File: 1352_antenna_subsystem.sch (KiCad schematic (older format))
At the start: 24 parts

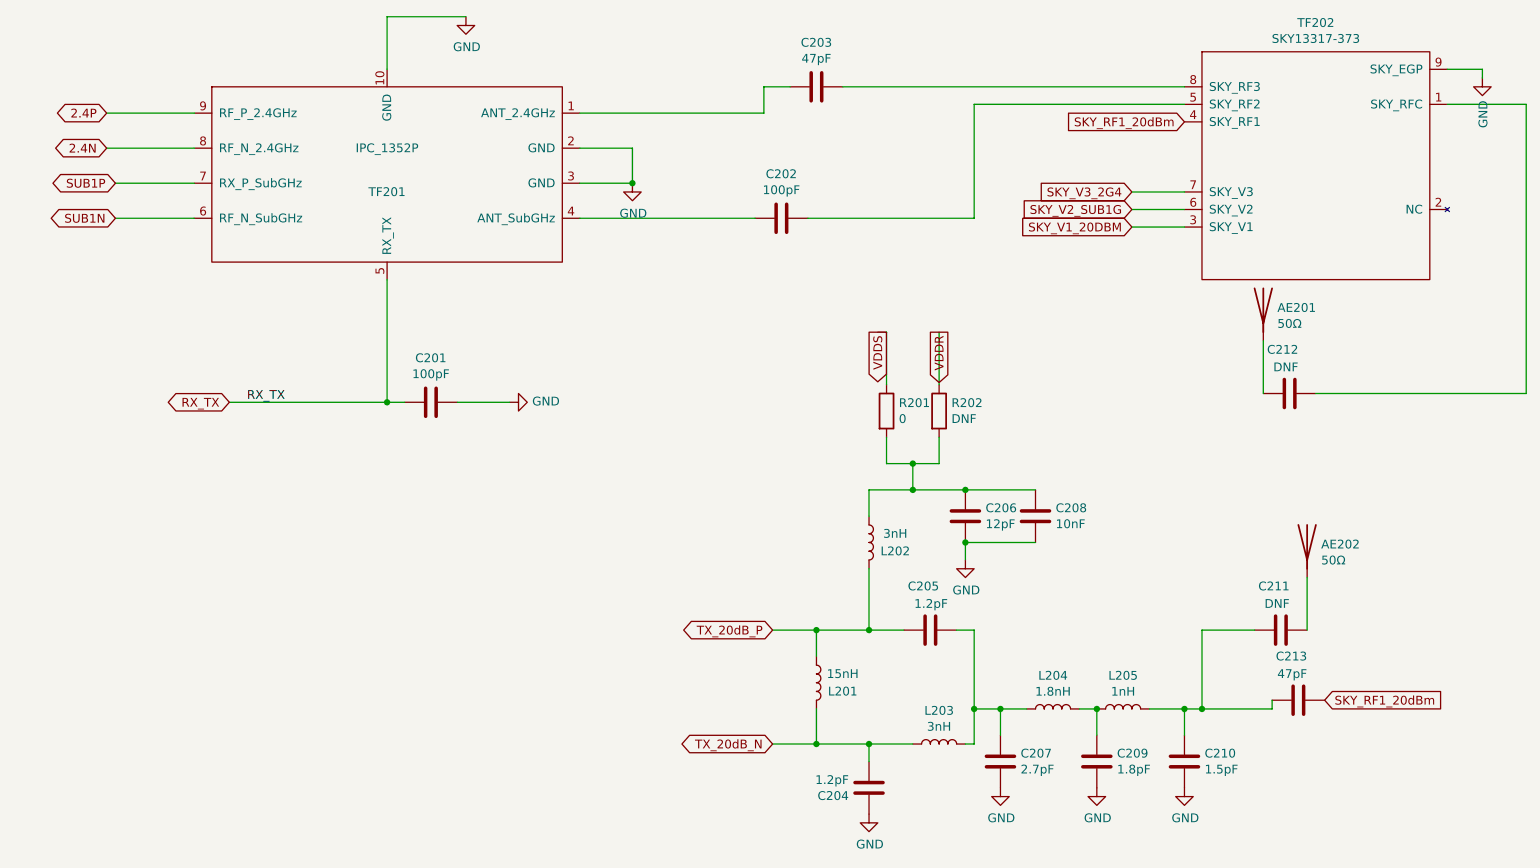
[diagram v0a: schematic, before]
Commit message: final edits before it'll be untouched
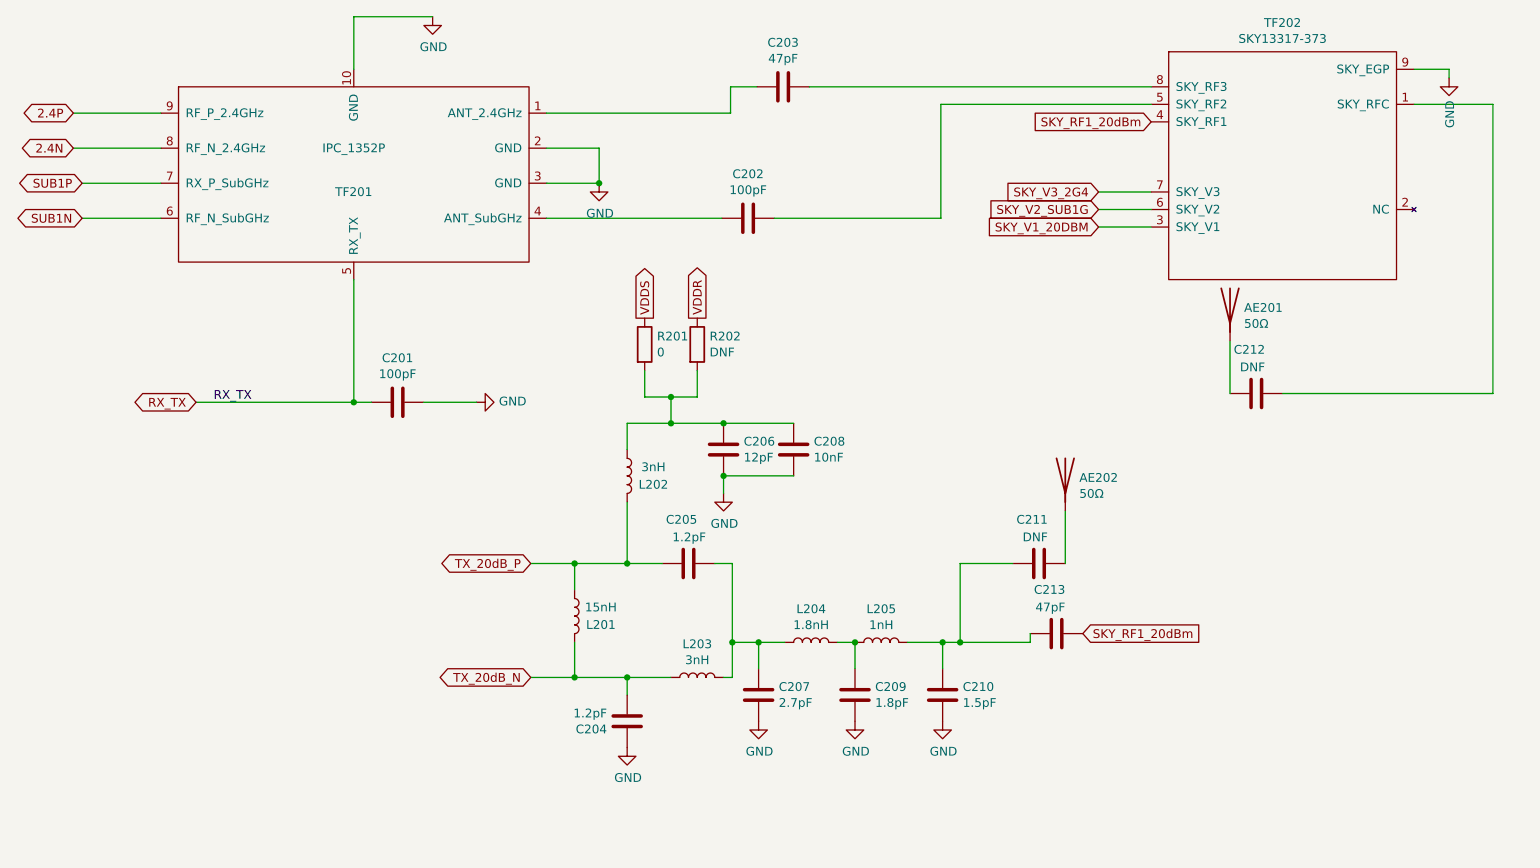
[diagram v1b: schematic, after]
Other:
- moved on the sheet: AE201, AE202, C201, C202, C203, C204, C205, C206, C207, C208, C209, C210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
